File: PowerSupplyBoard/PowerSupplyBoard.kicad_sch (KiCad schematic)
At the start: 76 parts, among them J101 BATTERY, J102 DATA2, J103 USB_C, J104 PWR, J105 DATA1, J106 USB_B_Micro, Q101 BSH205G2A, Q102 TD6790, Q103 TD6790, Q104 TD6790, SW101 SW_SPDT, U101 TPS63021, U102 MCP73834T, U103 TC7662Bx0A, U104 TC7662Bx0A, U105 CS5173

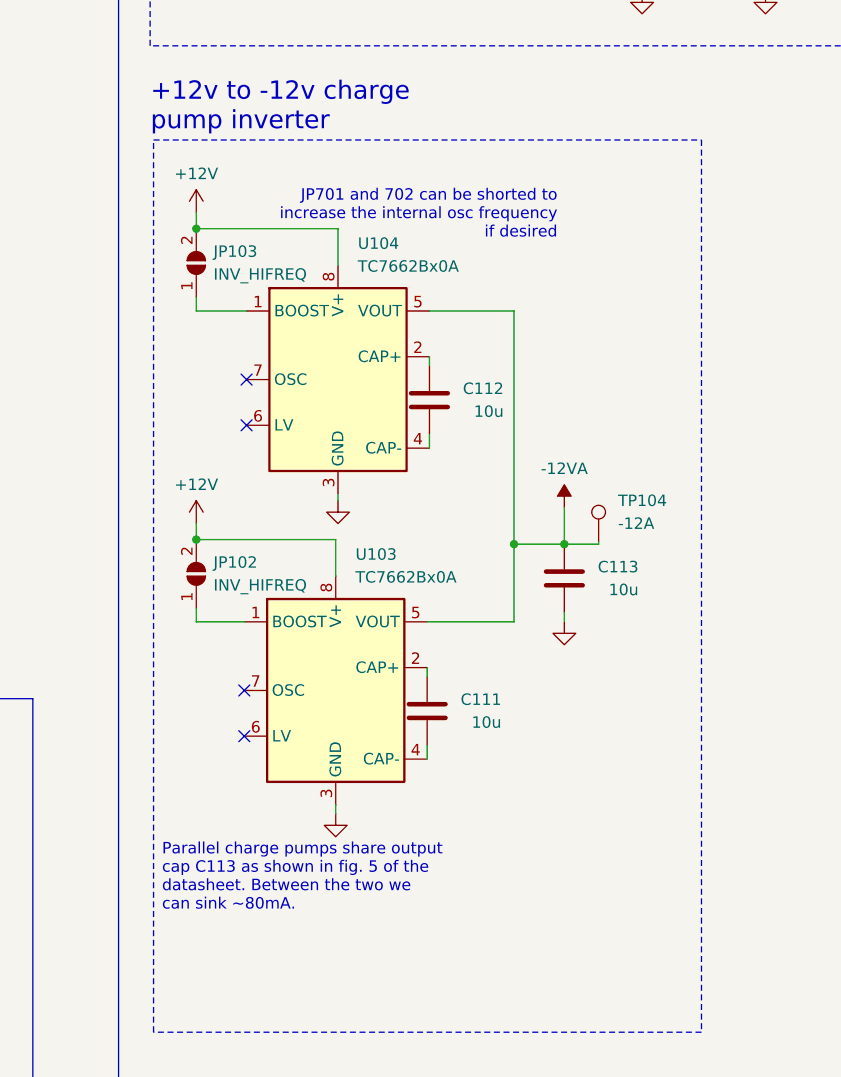
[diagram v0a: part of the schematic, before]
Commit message: AD5280 driver
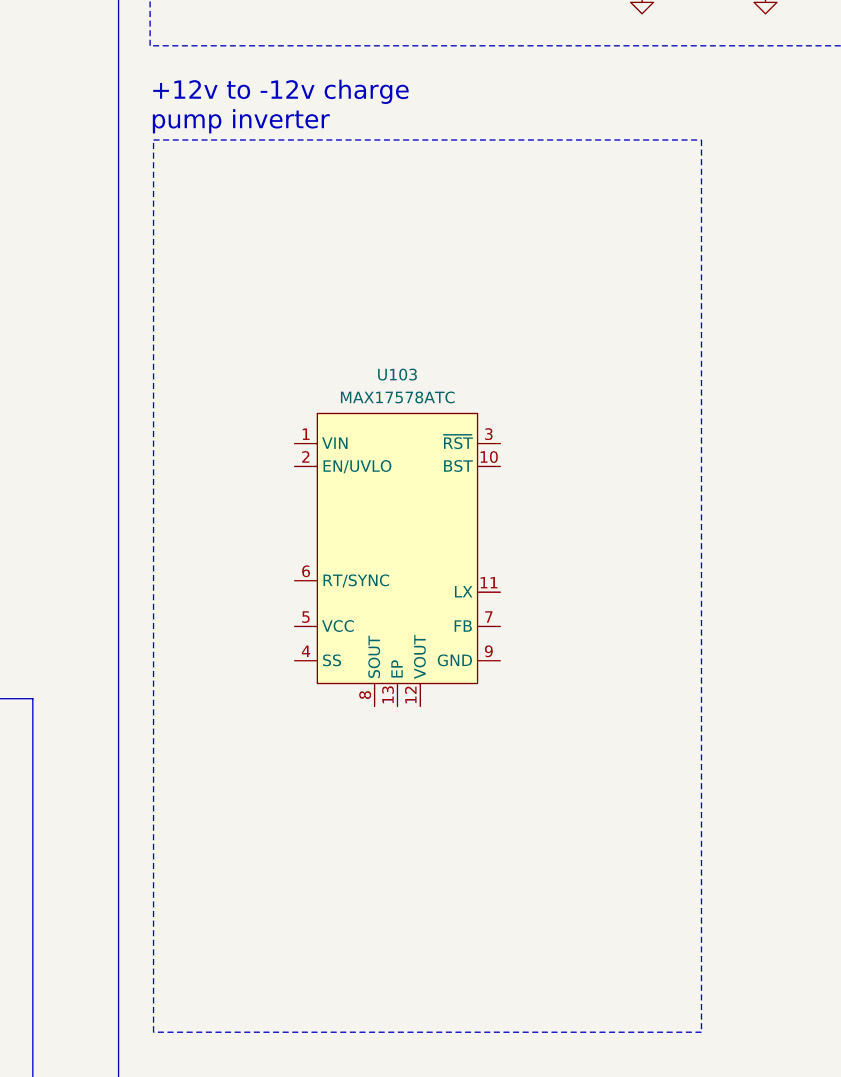
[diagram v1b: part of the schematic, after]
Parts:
- removed C111, C112, C113: 10u, Capacitor_SMD:C_0805_2012Metric, symbol Device:C
- removed JP102, JP103: INV_HIFREQ, Jumper:SolderJumper-2_Open_TrianglePad_0805, symbol Jumper:SolderJumper_2_Open
- removed TP104: -12A, TestPoint:TestPoint_Pad_D1.0mm_Value, symbol Connector:TestPoint
- removed U103, U104: TC7662Bx0A, Package_DIP:DIP-8_W7.62mm, symbol Converter_DCDC:TC7662Bx0A
- added U103: MAX17578ATC, Package_DFN_QFN:TDFN-12-1EP_3x3mm_P0.4mm_EP1.7x2.45mm, symbol Regulator_Switching:MAX17578ATC
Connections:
- no-connect marks 9 -> 5
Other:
- note removed: "JP701 and 702 can be shorted to increase the internal osc frequency if desired"
- note removed: "Parallel charge pumps share output cap C113 as shown in fig. 5 of the datasheet. Between the two we can sink ~80mA."

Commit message: Power board rev 3
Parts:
- removed C117, C118: 1u, Capacitor_SMD:C_0805_2012Metric, symbol Device:C
- removed C119, C120: 100n, Capacitor_SMD:C_0805_2012Metric, symbol Device:C
- removed D108: PMEG3030, Diode_SMD:D_SOD-123, symbol Device:D_Schottky
- removed D110: SP0503BAHT, Package_TO_SOT_SMD:SOT-143, symbol Power_Protection:SP0503BAHT
- removed J102: DATA2, Connector_PinHeader_2.54mm:PinHeader_1x02_P2.54mm_Vertical, symbol Connector:Conn_01x02_Pin
- removed J106: USB_B_Micro, Connector_USB:USB_Micro-B_Amphenol_10118193-0001LF_Horizontal, symbol Connector:USB_B_Micro
- removed JP101: DIG_CM, Jumper:SolderJumper-2_Open_TrianglePad_0805, symbol Jumper:SolderJumper_2_Open
- removed JP104: POS_CM, Jumper:SolderJumper-2_Open_TrianglePad_0805, symbol Jumper:SolderJumper_2_Open
- removed JP105: NEG_CM, Jumper:SolderJumper-2_Open_TrianglePad_0805, symbol Jumper:SolderJumper_2_Open
- removed Q102, Q103, Q104: TD6790, PCM_4ms_Package_SOIC:SM-8, symbol Transistor_BJT:TD6790
- removed TP106: -12V, TestPoint:TestPoint_Pad_D1.0mm_Value, symbol Connector:TestPoint
- removed TP107: +12V, TestPoint:TestPoint_Pad_D1.0mm_Value, symbol Connector:TestPoint
- added C111: 4u7, Capacitor_SMD:C_0805_2012Metric, symbol Device:C
- added C112: 4n7, Capacitor_SMD:C_0805_2012Metric, symbol Device:C
- added C113: 2u2, Capacitor_SMD:C_0805_2012Metric, symbol Device:C
- added L103: 22uH, Inductor_SMD:L_Changjiang_FNR4010S, symbol Device:L
- added R116: 330k, Resistor_SMD:R_0805_2012Metric, symbol Device:R_US
- added R117: 100k, Resistor_SMD:R_0805_2012Metric, symbol Device:R_US
- added RV101, RV102: 10k, Potentiometer_THT:Potentiometer_Bourns_3296W_Vertical, symbol Device:R_Potentiometer_Trim_US
- C103: value 22u -> 100n
- C107: value 100n -> 22u
- R103: value 10k -> 1k
- R111: value 4k7 -> 470k
- R112: value 12k -> 33k
- R113: value 12k -> 4k7
- TP101: value 3V3 -> -12
- TP102: value 3V3P -> 3V3
- TP105: value +12A -> +12
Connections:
- net +12V: now also C116.1, D106.1 (K), R110.1, TP105.1, U103.1 (VIN), C111.1, R116.1
- net +3.3V: now also C108.1, R105.1, R113.2, TP102.1, U101.3 (FB), U101.4 (VOUT), U101.5 (VOUT); no longer C107.1, TP101.1
- net -12V: now also C107.2, R112.2, TP101.1, U103.12 (VOUT), U103.13 (EP), U103.8 (SOUT), C112.2, C113.2
- net GND: now also C107.1, R103.2, R111.1, U103.9 (GND), C111.2, L103.2, R117.2; no longer C103.2, C107.2, R111.2
- net at U103.10 (BST): now also C103.1
- net at U103.11 (LX): now also C103.2, L103.1
- net at U103.2 (EN/UVLO): now also R116.2, R117.1
- net NRST: now reaches U103.3 (~{RST})
- net NRST: now also R113.1
- net at U103.4 (SS): now also C112.1
- net at U103.5 (VCC): now also C113.1
- net at U103.7 (FB): now also R111.2, RV102.1
- net at R110.2, U105.2 (FB): now also RV101.1; no longer R111.1
- removed net +12VA: C116.1, D106.1 (K), R110.1, R113.1, TP105.1
- removed net +3.3VP: C108.1, R103.1, R105.1, TP102.1, U101.3 (FB), U101.4 (VOUT), U101.5 (VOUT)
- net -12VA: no longer names the net of R112.1
- net -12VA: now also RV102.2, RV102.3
- new net: R103.1, RV101.2, RV101.3
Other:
- note added: "USB Connector"
- note removed: "BJT capacitance multipliers"
- note removed: "These capacitance multipliers should smooth the power lines to <1mV of ripple when populated, if not they can be bypassed with solder jumpers"
- note removed: "USB Connectors"
- moved on the sheet: C101, C102, C104, C105, C106, C108, C109, C110, C114, C115, C116, D101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
